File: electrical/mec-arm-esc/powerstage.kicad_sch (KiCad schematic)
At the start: 12 parts, among them Q1 STL110N10F7, Q2 STL110N10F7, U1 L6387ED

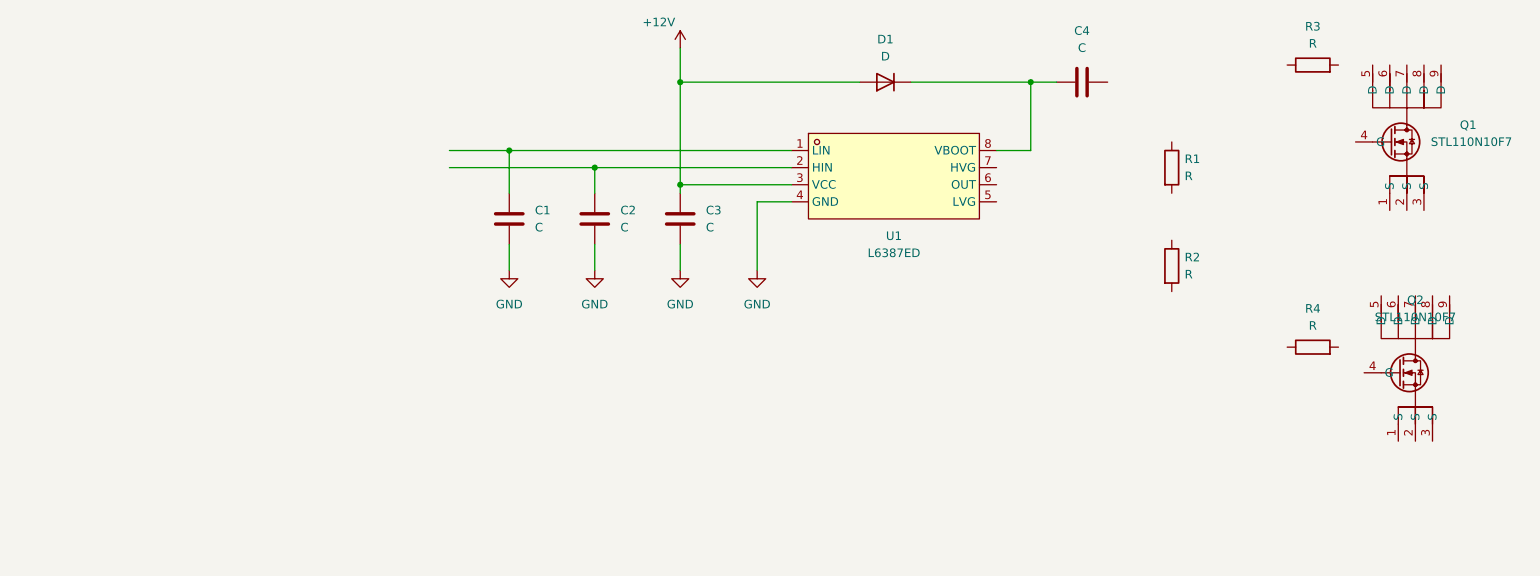
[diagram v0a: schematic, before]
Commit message: finish single phase
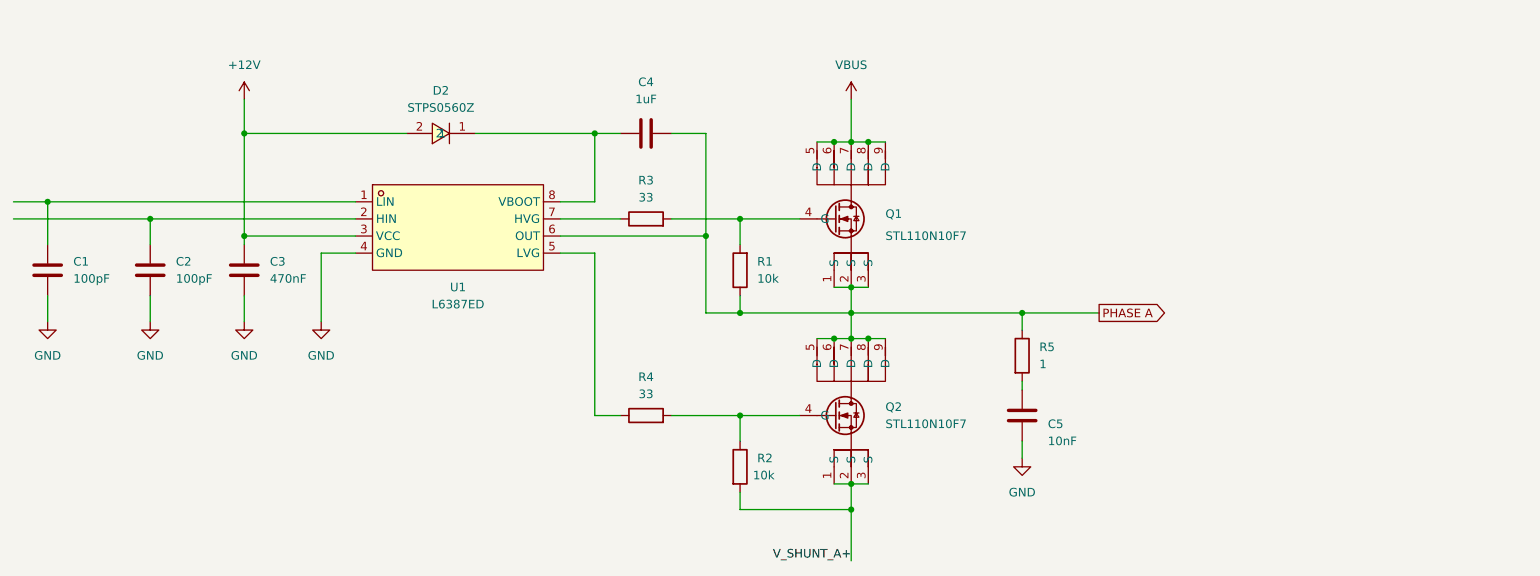
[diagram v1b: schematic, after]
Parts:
- removed D1: D, symbol Device:D
- added C5: 10nF, symbol Device:C
- added D2: STPS0560Z, EasyEDA:SOD-123_L2.7-W1.6-LS3.7-RD, symbol core:STPS0560Z
- added R5: 1, symbol Device:R
- C1, C2: value C -> 100pF
- C3: value C -> 470nF
- C4: value C -> 1uF
- R1, R2: value R -> 10k
- R3, R4: value R -> 33
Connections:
- net +12V: now also D2.2
- net GND: now also C5.1
- net at C4.1, U1.8 (VBOOT): now also D2.1
- net PHASE A: now reaches C4.2
- net PHASE A: now also Q1.1 (S), Q1.2 (S), Q1.3 (S), Q2.5 (D), Q2.6 (D), Q2.7 (D), Q2.8 (D), Q2.9 (D), R1.1, U1.6 (OUT), R5.1
- net V_SHUNT_A+: now reaches Q2.1 (S)
- net V_SHUNT_A+: now also Q2.2 (S), Q2.3 (S), R2.2
- net at Q2.4 (G): now also R2.1, R4.2
- net at U1.5 (LVG): now also R4.1
- net at U1.7 (HVG): now also R3.1
- net at Q1.4 (G): now also R1.2, R3.2
- net VBUS: now reaches Q1.5 (D)
- net VBUS: now also Q1.6 (D), Q1.7 (D), Q1.8 (D), Q1.9 (D)
- new net: C5.2, R5.2
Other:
- moved on the sheet: C1, C2, C3, C4, Q1, Q2, R1, R2, R3, R4, U1
